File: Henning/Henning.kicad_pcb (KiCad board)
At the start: 2 copper layers, 68 x 38 mm, 19 parts, among them P1 RS232, P2 EBUS, Q1 BD645, U1 4011, U2 CNY17-1, U3 78L05, U4 CNY17-1

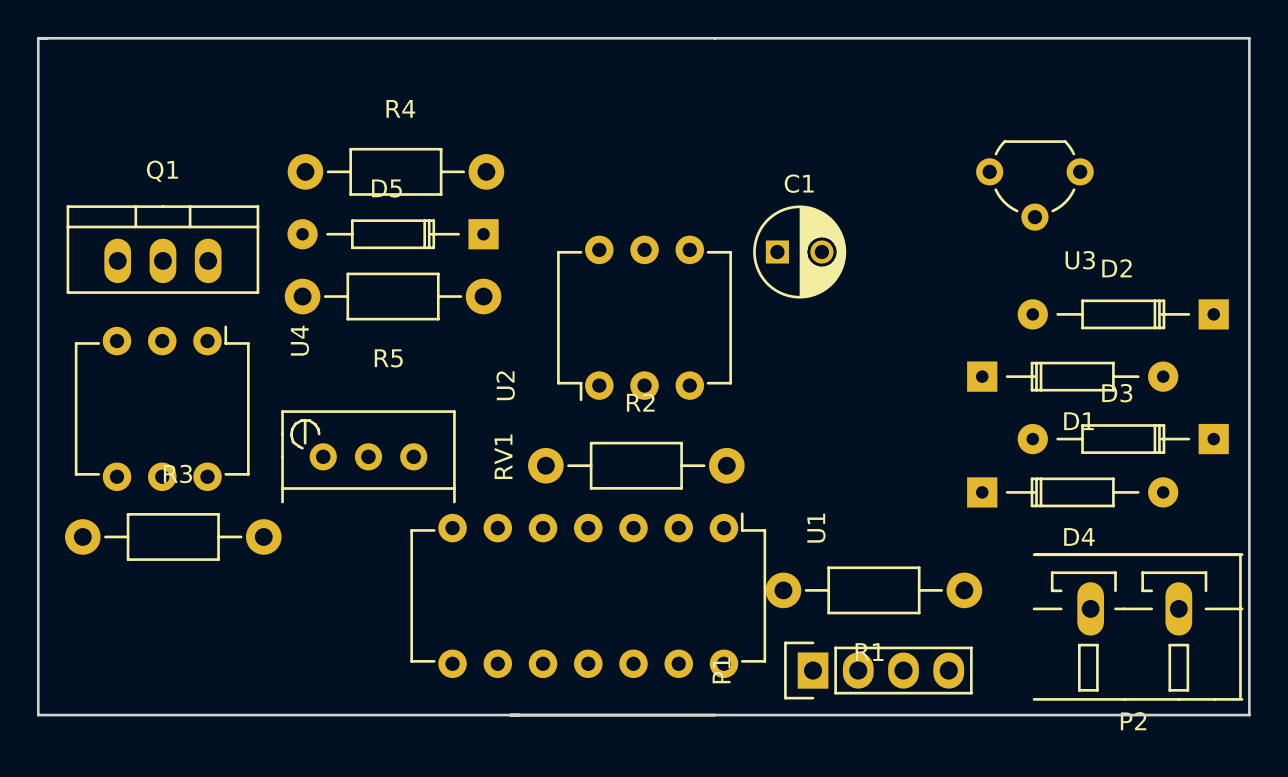
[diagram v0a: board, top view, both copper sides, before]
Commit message: Fixed PCB
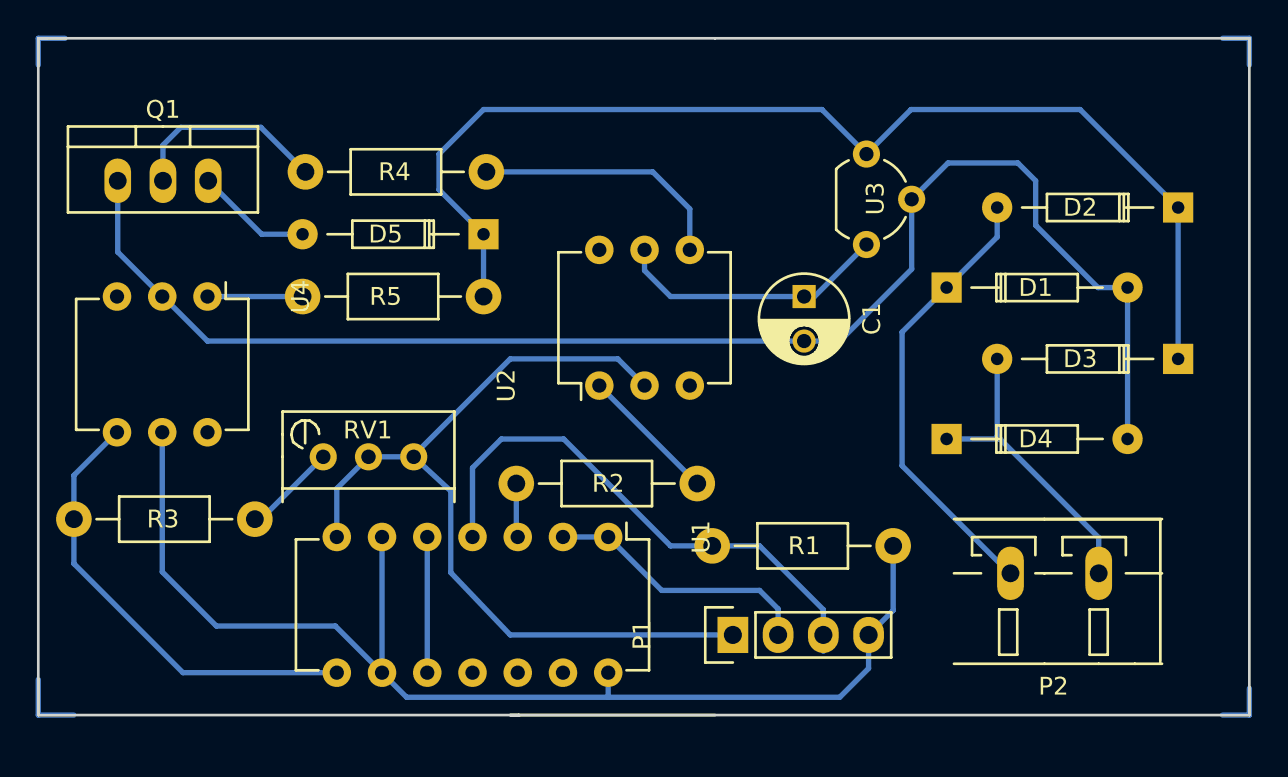
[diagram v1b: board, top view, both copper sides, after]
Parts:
- D1, D2, D3, D4: value D -> 1N4148
- moved U3 12.0 mm to (58.5, 18.5), turned to 270 degrees
- moved R2 8.56 mm to (49.0, 37.0), turned to 180 degrees
- moved U1 6.52 mm to (44.0, 40.0)
- moved D2 6.32 mm to (76.0, 21.5)
- moved D1 5.39 mm to (63.0, 26.0)
- moved D3 4.92 mm to (76.0, 30.0)
- moved P1 4.92 mm to (51.0, 45.5)
- moved P2 4.92 mm to (69.0, 39.5)
- moved R1 4.72 mm to (60.0, 40.5)
- moved Q1 4.50 mm to (19.0, 20.0)
- moved D4 3.61 mm to (63.0, 34.5)
- moved C1 2.92 mm to (55.0, 26.5), turned to 270 degrees
- moved U4 2.50 mm to (21.5, 26.5)
- moved R3 1.12 mm to (14.0, 39.0)
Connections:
- D1 pad 1: Net-(C1-Pad2) -> EBUS1
- D1 pad 2: EBUS1 -> Net-(C1-Pad2)
- D2 pad 1: EBUS1 -> Net-(D2-Pad1)
- D2 pad 2: Net-(D2-Pad2) -> EBUS1
- D3 pad 1: EBUS2 -> Net-(D2-Pad1)
- D3 pad 2: Net-(D2-Pad2) -> EBUS2
- D4 pad 1: Net-(C1-Pad2) -> EBUS2
- D4 pad 2: EBUS2 -> Net-(C1-Pad2)
- D5 pad 1: Net-(D2-Pad2) -> Net-(D2-Pad1)
- R5 pad 1: Net-(D2-Pad2) -> Net-(D2-Pad1)
- U3 pad 1: Net-(D2-Pad2) -> Net-(D2-Pad1)
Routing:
- net Net-(C1-Pad2): track 0.00 -> 82.1 mm
- net VDD: track 0.00 -> 67.7 mm
- net Net-(D2-Pad1): track 0.00 -> 64.4 mm
- net GND: track 0.00 -> 48.5 mm
- net RXD: track 0.00 -> 30.6 mm
- net Net-(R3-Pad1): track 0.00 -> 25.7 mm
- net EBUS1: track 0.00 -> 25.3 mm
- net EBUS2: track 0.00 -> 17.4 mm
- net Net-(C1-Pad1): track 0.00 -> 15.4 mm
- net TXD: track 0.00 -> 15.2 mm
- net Net-(R4-Pad2): track 0.00 -> 14.6 mm
- net (no net): track 0.00 -> 13.0 mm
- net Net-(Q1-Pad2): track 0.00 -> 11.4 mm
- net Net-(R2-Pad1): track 0.00 -> 7.78 mm
- net Net-(U1-Pad10): track 0.00 -> 7.62 mm
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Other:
- net class Default: trace_width 0.25 -> 0.3
